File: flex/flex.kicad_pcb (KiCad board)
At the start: 2 copper layers, 126.3 x 113 mm, 105 parts, among them J1 Conn_01x06_Female, J2 Conn_01x05_Female, J3 Conn_01x03_Female, J4 Conn_01x06_Female, J5 Conn_01x03_Female, SW1 SW_Push, SW10 SW_Push, SW11 SW_Push, SW12 SW_Push, SW14 SW_Push, SW15 SW_Push, SW16 SW_Push, SW17 SW_Push, SW19 SW_Push, SW2 SW_Push, SW20 SW_Push, SW21 SW_Push, SW22 SW_Push, SW23 SW_Push, SW24 SW_Push, SW25 SW_Push, SW26 SW_Push, SW3 SW_Push, SW4 SW_Push, SW5 SW_Push, SW6 SW_Push, SW7 SW_Push, SW8 SW_Push, SW9 SW_Push

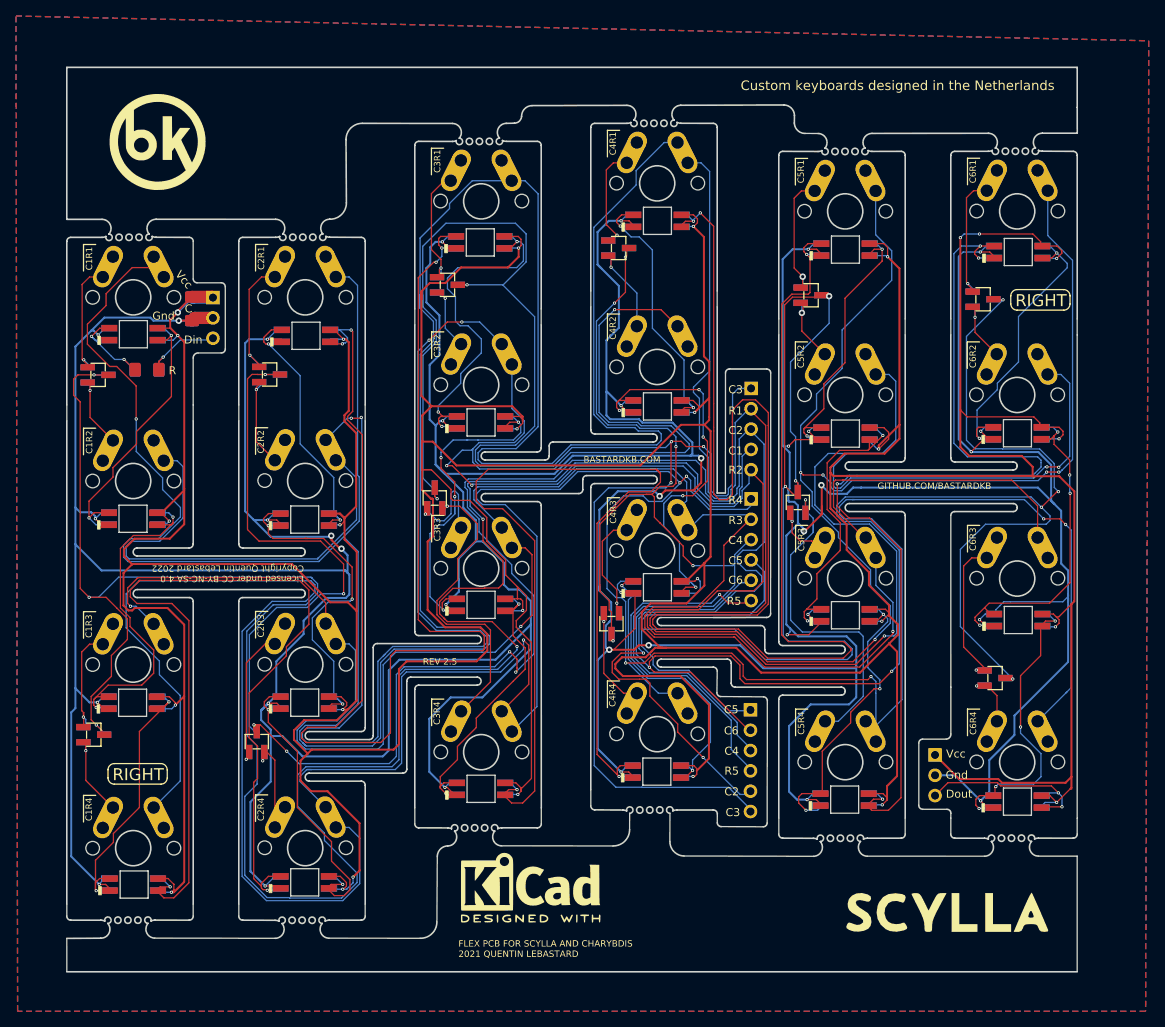
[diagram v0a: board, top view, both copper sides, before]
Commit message: edge cuts, via size
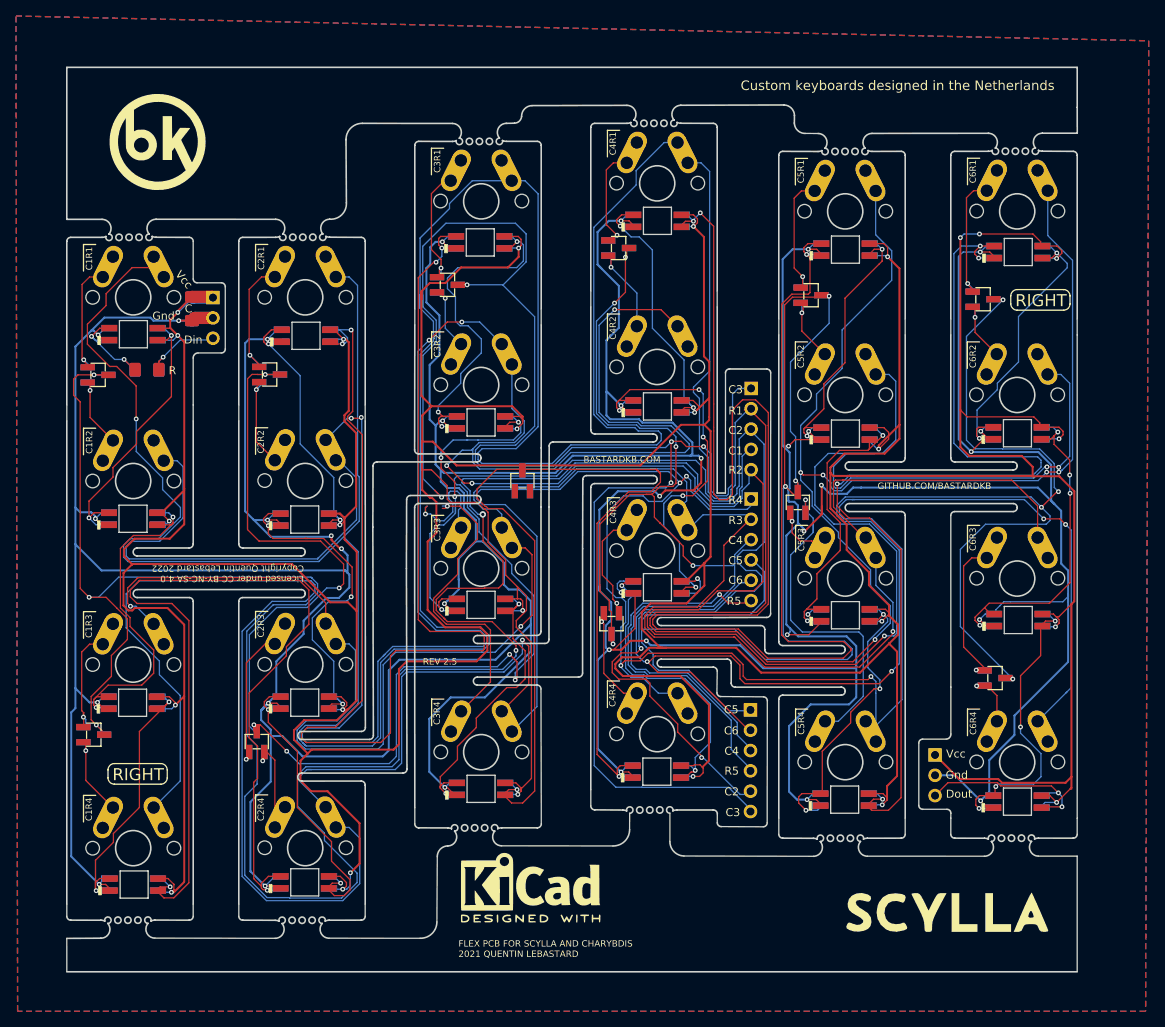
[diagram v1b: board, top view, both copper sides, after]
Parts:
- moved D10 11.2 mm to (92.4, 78.3)
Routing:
- net col1: track 286.2 -> 288.9 mm
- net col2: track 273.9 -> 276.4 mm
- net row4: track 431.6 -> 433.8 mm
- net Vcc: track 930.8 -> 933.0 mm
- net Net-(D37-Pad1): track 38.3 -> 40.1 mm
- net col4: track 132.9 -> 134.7 mm
- net Net-(D10-Pad2): track 14.1 -> 15.1 mm
- net row5: track 45.7 -> 46.7 mm
- net Net-(D25-Pad1): track 125.9 -> 125.0 mm
- net row3: track 263.9 -> 264.7 mm
- net Net-(D23-Pad1): track 38.2 -> 38.9 mm
- net Net-(D5-Pad1): track 40.3 -> 39.8 mm
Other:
- outline, holes or cut-outs redrawn
